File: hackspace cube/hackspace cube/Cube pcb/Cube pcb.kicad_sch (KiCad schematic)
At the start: 57 parts, among them J1 Conn_01x08 ( conector 1), J2 Conn_01x08 ( conector 2), J3 Conn_01x02 ( exstra ground co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, J4 Conn_01x14 ( Spare Ports ), Q1 BSS138, Q10 BSS138, Q11 BSS138, Q12 BSS138, Q13 BSS138, Q14 BSS138, Q15 BSS138, Q16 BSS138, Q2 BSS138, Q3 BSS138, Q4 BSS138, Q5 BSS138, Q6 BSS138, Q7 BSS138, Q8 BSS138, Q9 BSS138

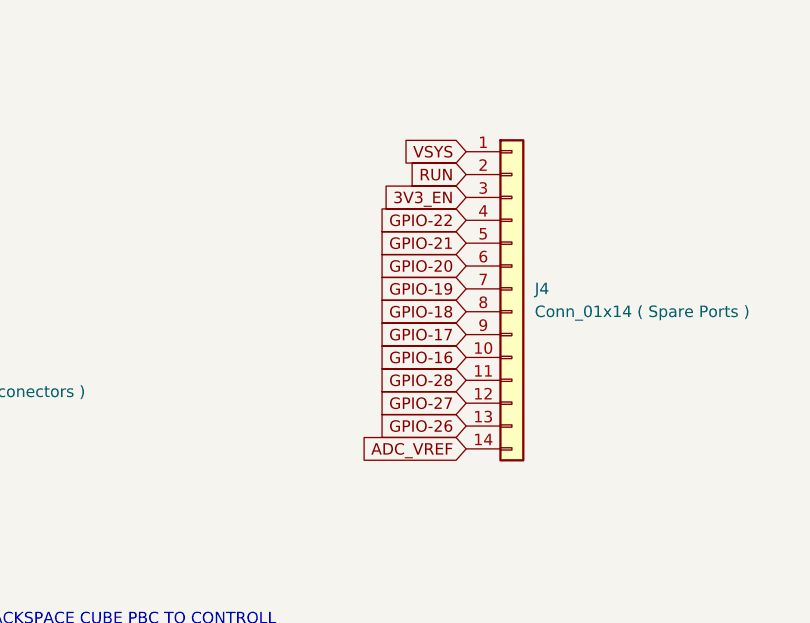
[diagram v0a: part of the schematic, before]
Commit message: pcb first draft
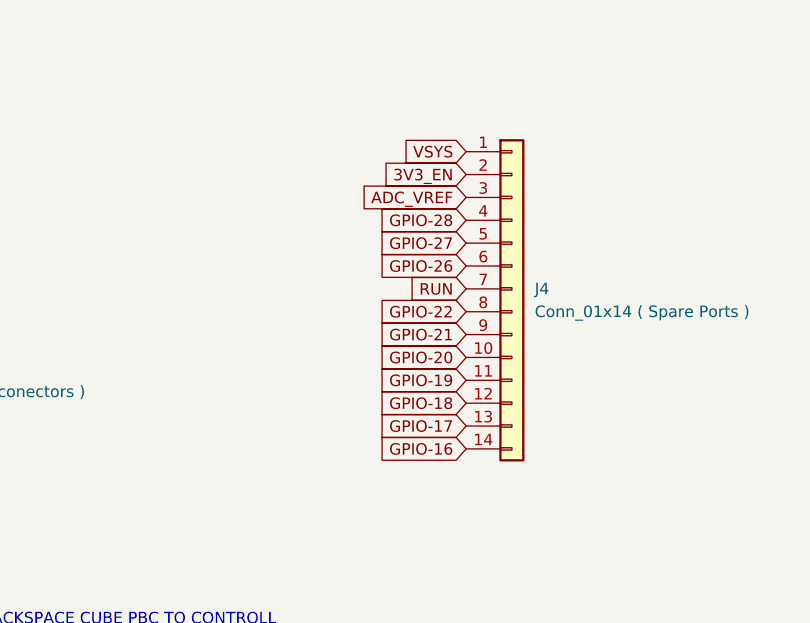
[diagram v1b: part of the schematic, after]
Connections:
- net 3V3_EN: now also J4.2 (Pin_2); no longer J4.3 (Pin_3)
- net ADC_VREF: now also J4.3 (Pin_3); no longer J4.14 (Pin_14)
- net GPIO-16: now also J4.14 (Pin_14); no longer J4.10 (Pin_10)
- net GPIO-17: now also J4.13 (Pin_13); no longer J4.9 (Pin_9)
- net GPIO-18: now also J4.12 (Pin_12); no longer J4.8 (Pin_8)
- net GPIO-19: now also J4.11 (Pin_11); no longer J4.7 (Pin_7)
- net GPIO-20: now also J4.10 (Pin_10); no longer J4.6 (Pin_6)
- net GPIO-21: now also J4.9 (Pin_9); no longer J4.5 (Pin_5)
- net GPIO-22: now also J4.8 (Pin_8); no longer J4.4 (Pin_4)
- net GPIO-26: now also J4.6 (Pin_6); no longer J4.13 (Pin_13)
- net GPIO-27: now also J4.5 (Pin_5); no longer J4.12 (Pin_12)
- net GPIO-28: now also J4.4 (Pin_4); no longer J4.11 (Pin_11)
- net RUN: now also J4.7 (Pin_7); no longer J4.2 (Pin_2)
